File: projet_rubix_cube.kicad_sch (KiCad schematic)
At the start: 14 parts, among them J1 Screw_Terminal_01x04, J2 Screw_Terminal_01x04, J3 Screw_Terminal_01x03, U2 L298HN

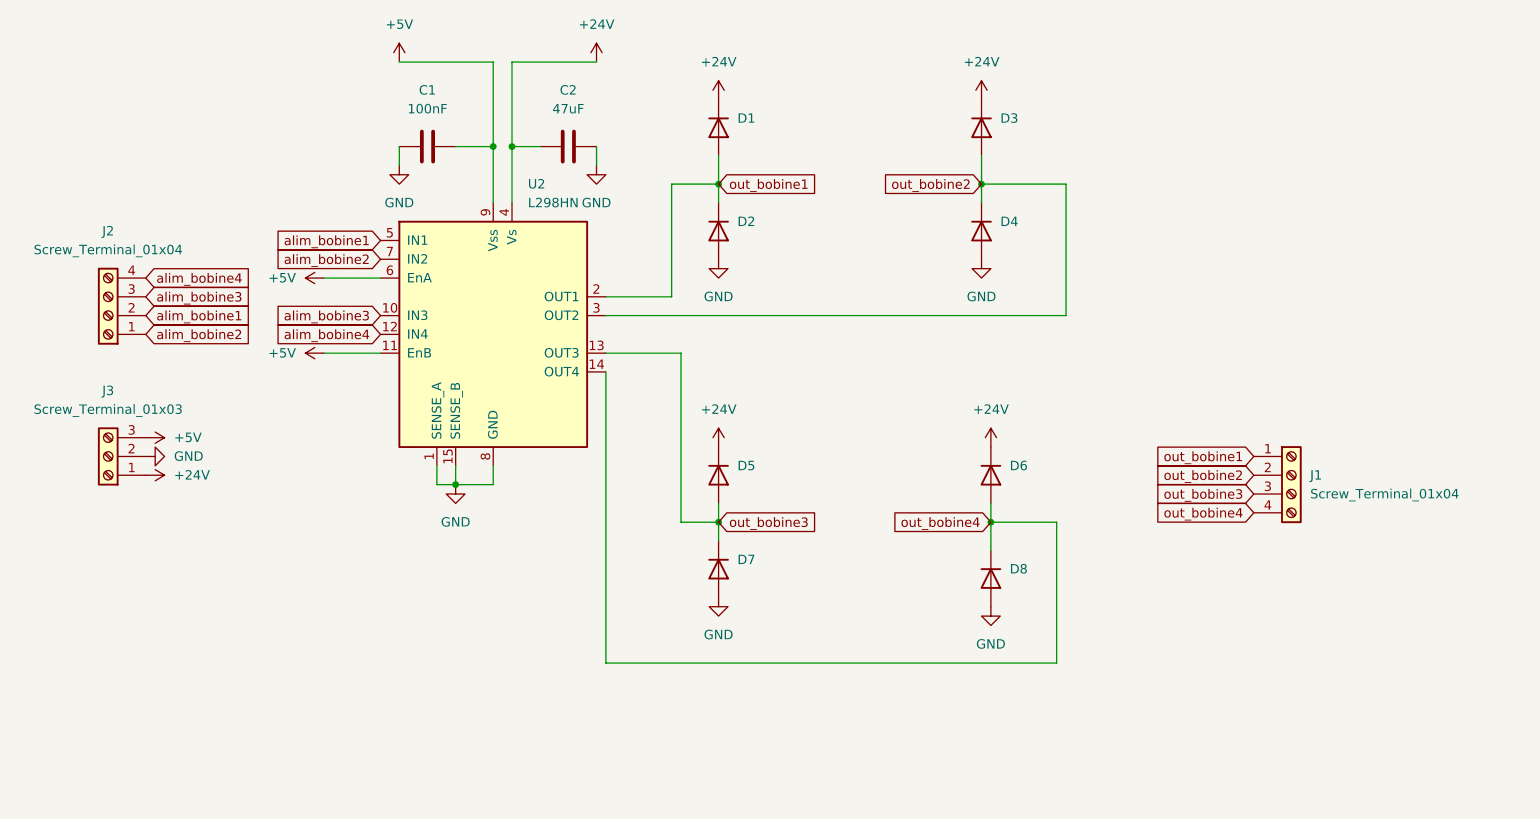
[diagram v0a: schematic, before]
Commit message: Push update schematic & PCB
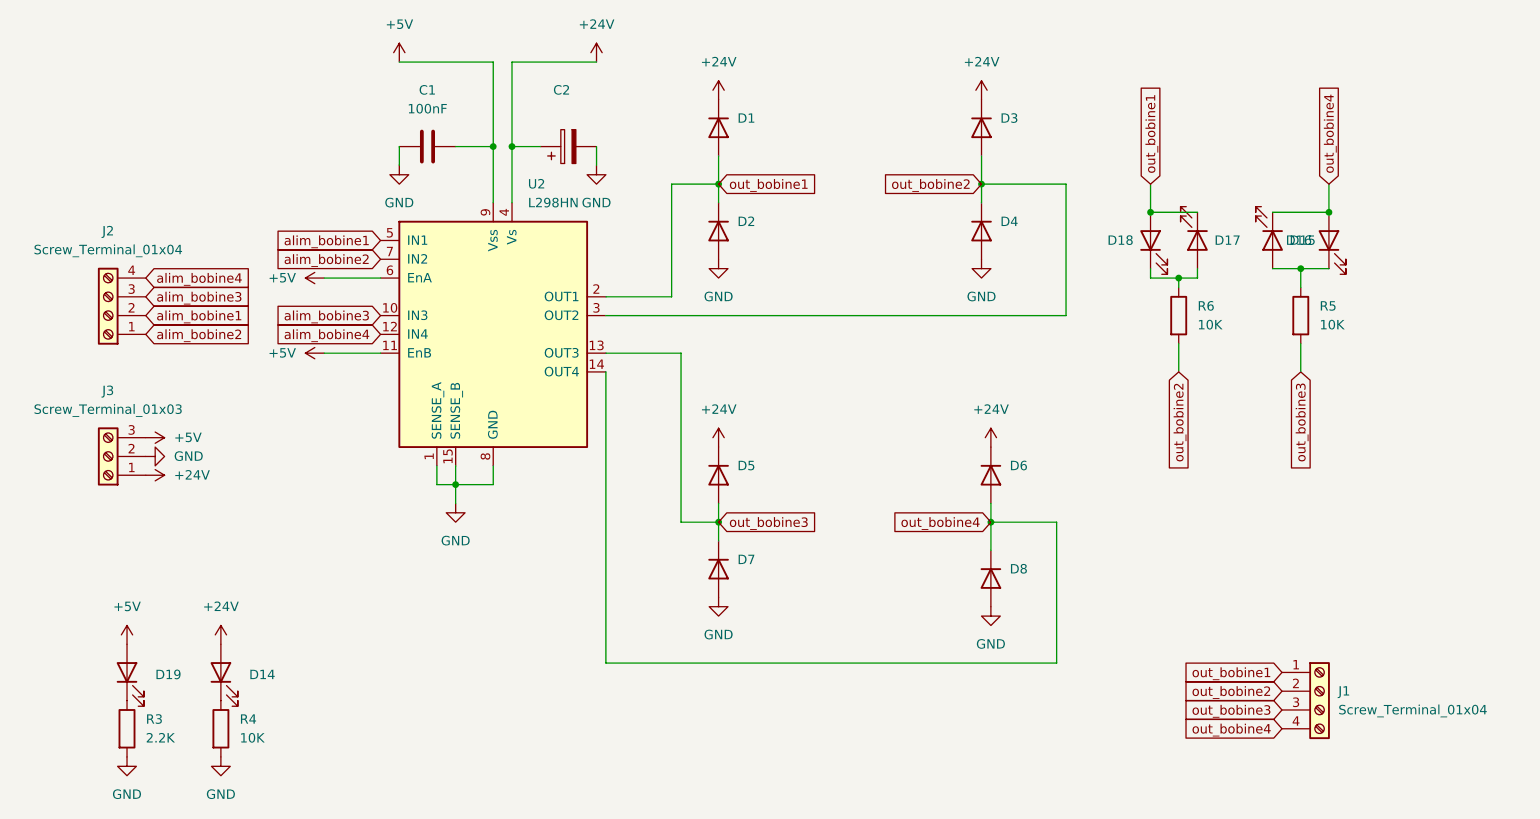
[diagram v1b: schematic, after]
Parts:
- removed C2: 47uF, Capacitor_SMD:C_0805_2012Metric, symbol Device:C
- added C2: (no value), Capacitor_SMD:C_Elec_6.3x7.7, symbol Device:C_Polarized
- added D14, D19: LED_Yellow, LED_SMD:LED_0603_1608Metric, symbol Device:LED
- added D15, D16, D17, D18: LED_Blue, LED_SMD:LED_0603_1608Metric, symbol Device:LED
- added R3: 2.2K, Resistor_SMD:R_0603_1608Metric, symbol Device:R
- added R4, R5, R6: 10K, Resistor_SMD:R_0603_1608Metric, symbol Device:R
- C1: footprint Capacitor_SMD:C_0201_0603Metric -> Capacitor_SMD:C_0603_1608Metric; LCSC (none) -> C14663
- D1, D2, D3, D4, D5, D6, D7, D8: footprint Diode_SMD:D_SOD-323F -> Diode_SMD:D_SOD-323; LCSC (none) -> C191023
- J1, J2: footprint Connector_PinHeader_1.00mm:PinHeader_1x04_P1.00mm_Horizontal -> Connector_PinHeader_1.00mm:PinHeader_1x04_P1.00mm_Vertical
- J3: footprint Connector_PinHeader_1.00mm:PinHeader_1x03_P1.00mm_Horizontal -> Connector_PinHeader_1.00mm:PinHeader_1x03_P1.00mm_Vertical
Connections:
- net +24V: now also C2.1, D14.2 (A)
- net +5V: now also D19.2 (A)
- net GND: now also C2.2, R3.2, R4.2
- net out_bobine1: now also D17.1 (K), D18.2 (A)
- net out_bobine2: now also R6.2
- net out_bobine3: now also R5.2
- net out_bobine4: now also D15.1 (K), D16.2 (A)
- new net: D17.2 (A), D18.1 (K), R6.1
- new net: D15.2 (A), D16.1 (K), R5.1
- new net: D14.1 (K), R4.1
- new net: D19.1 (K), R3.1
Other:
- moved on the sheet: J1

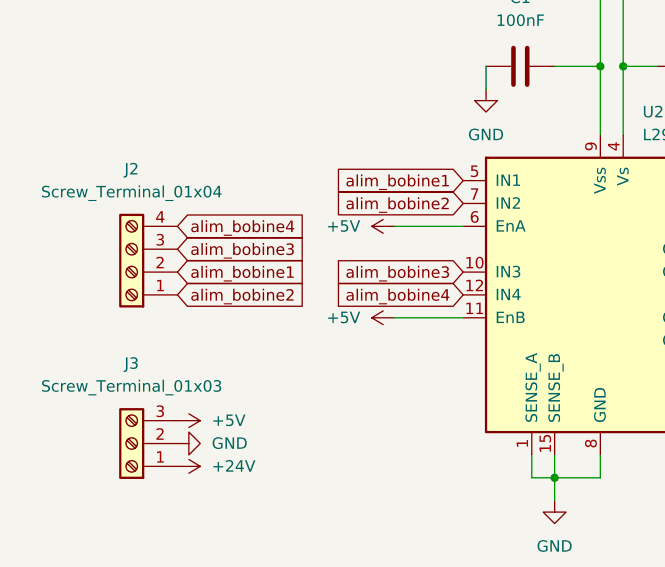
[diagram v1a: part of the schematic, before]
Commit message: routage_carte
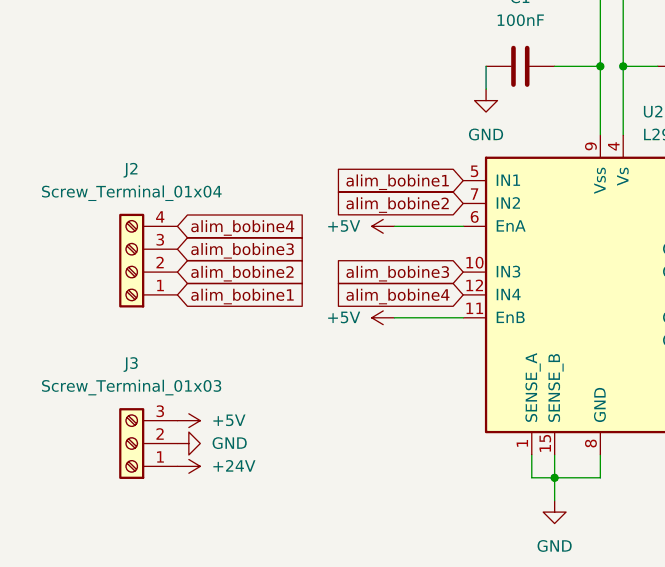
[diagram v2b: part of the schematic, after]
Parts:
- C2: value (none) -> ~
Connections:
- net alim_bobine1: now also J2.1 (Pin_1); no longer J2.2 (Pin_2)
- net alim_bobine2: now also J2.2 (Pin_2); no longer J2.1 (Pin_1)
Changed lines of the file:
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@@
 	(global_label "alim_bobine2"
 		(shape input)
-		(at 96.52 66.04 0)
+		(at 96.52 63.5 0)
 		(fields_autoplaced yes)
 		(effects
@@
 		)
 		(property "Intersheetrefs" "${INTERSHEET_REFS}"
-			(at 112.084 66.04 0)
+			(at 112.084 63.5 0)
 			(effects
 				(font
@@
 	(global_label "alim_bobine1"
 		(shape input)
-		(at 96.52 63.5 0)
+		(at 96.52 66.04 0)
 		(fields_autoplaced yes)
 		(effects
@@
 		)
 		(property "Intersheetrefs" "${INTERSHEET_REFS}"
-			(at 112.084 63.5 0)
+			(at 112.084 66.04 0)
 			(effects
 				(font
@@
 			)
 		)
-		(property "Value" ""
+		(property "Value" "~"
 			(at 152.781 35.56 90)
 			(effects

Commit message: DRC OK
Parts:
- J1, J2: footprint Connector_PinHeader_1.00mm:PinHeader_1x04_P1.00mm_Vertical -> Connector_PinHeader_2.54mm:PinHeader_1x04_P2.54mm_Vertical
- J3: footprint Connector_PinHeader_1.00mm:PinHeader_1x03_P1.00mm_Vertical -> Connector_PinSocket_2.54mm:PinSocket_1x03_P2.54mm_Vertical
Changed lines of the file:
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@@
 			)
 		)
-		(property "Footprint" "Connector_PinHeader_1.00mm:PinHeader_1x03_P1.00mm_Vertical"
+		(property "Footprint" "Connector_PinSocket_2.54mm:PinSocket_1x03_P2.54mm_Vertical"
 			(at 91.44 82.55 0)
 			(effects
@@
 			)
 		)
-		(property "Footprint" "Connector_PinHeader_1.00mm:PinHeader_1x04_P1.00mm_Vertical"
+		(property "Footprint" "Connector_PinHeader_2.54mm:PinHeader_1x04_P2.54mm_Vertical"
 			(at 91.44 63.5 0)
 			(effects
@@
 			)
 		)
-		(property "Footprint" "Connector_PinHeader_1.00mm:PinHeader_1x04_P1.00mm_Vertical"
+		(property "Footprint" "Connector_PinHeader_2.54mm:PinHeader_1x04_P2.54mm_Vertical"
 			(at 255.27 114.3 0)
 			(effects

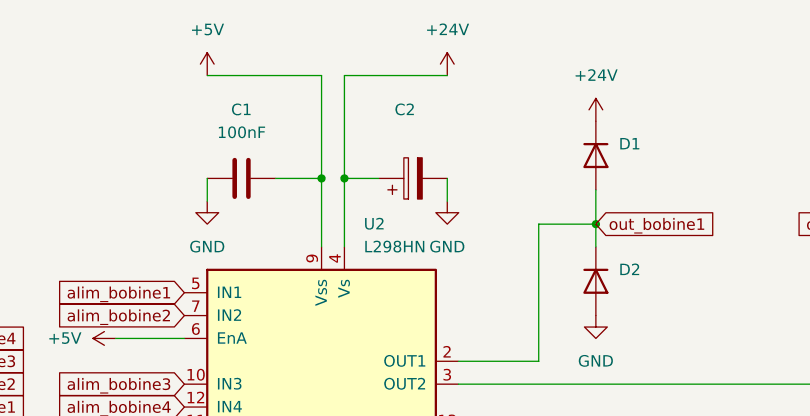
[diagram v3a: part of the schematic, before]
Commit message: alimentation DC/DC
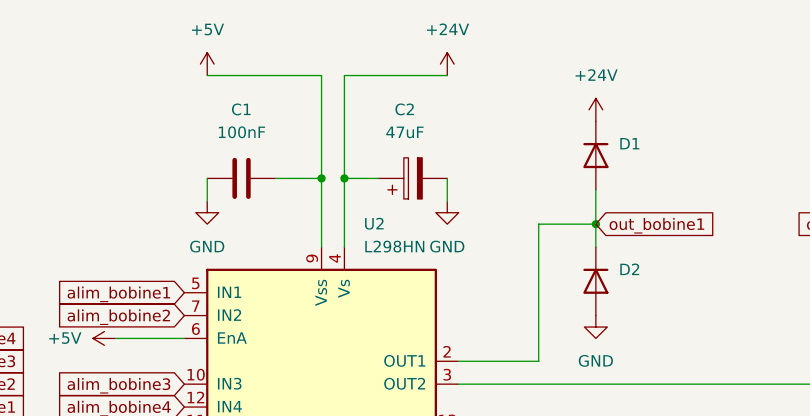
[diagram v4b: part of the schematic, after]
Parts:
- C2: value ~ -> 47uF
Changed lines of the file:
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@@
 			)
 		)
-		(property "Value" "~"
+		(property "Value" "47uF"
 			(at 152.781 35.56 90)
 			(effects
@@
 					(size 1.27 1.27)
 				)
-				(hide yes)
 			)
 		)
